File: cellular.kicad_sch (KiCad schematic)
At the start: 50 parts, among them J5 SIM8060-6-1-14-00-A, J6 Conn_Coaxial, J7 Conn_Coaxial, Q6 MMBT3904, Q7 MMBT3904, U24 SN74AXC4T245QPWRQ1, U25 SN74AXC4T245QPWRQ1, U26 BG95-M3

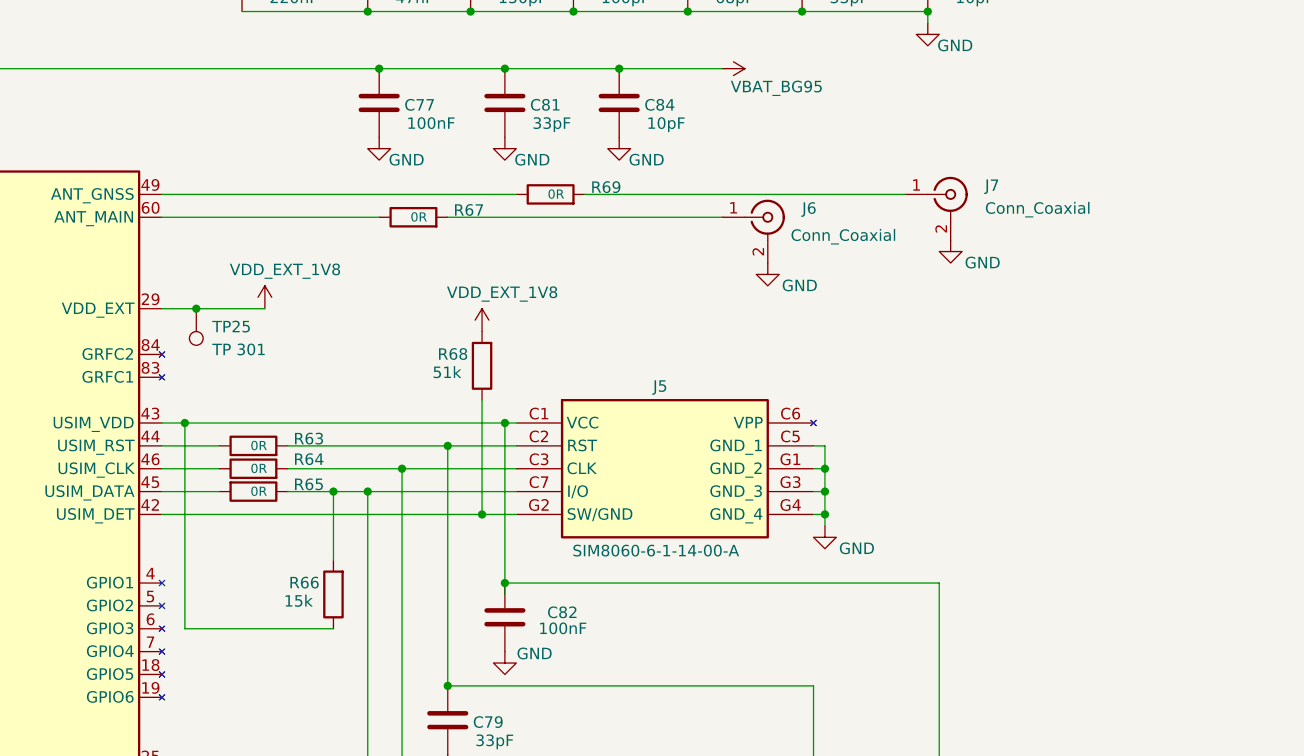
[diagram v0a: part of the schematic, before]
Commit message: bug fix
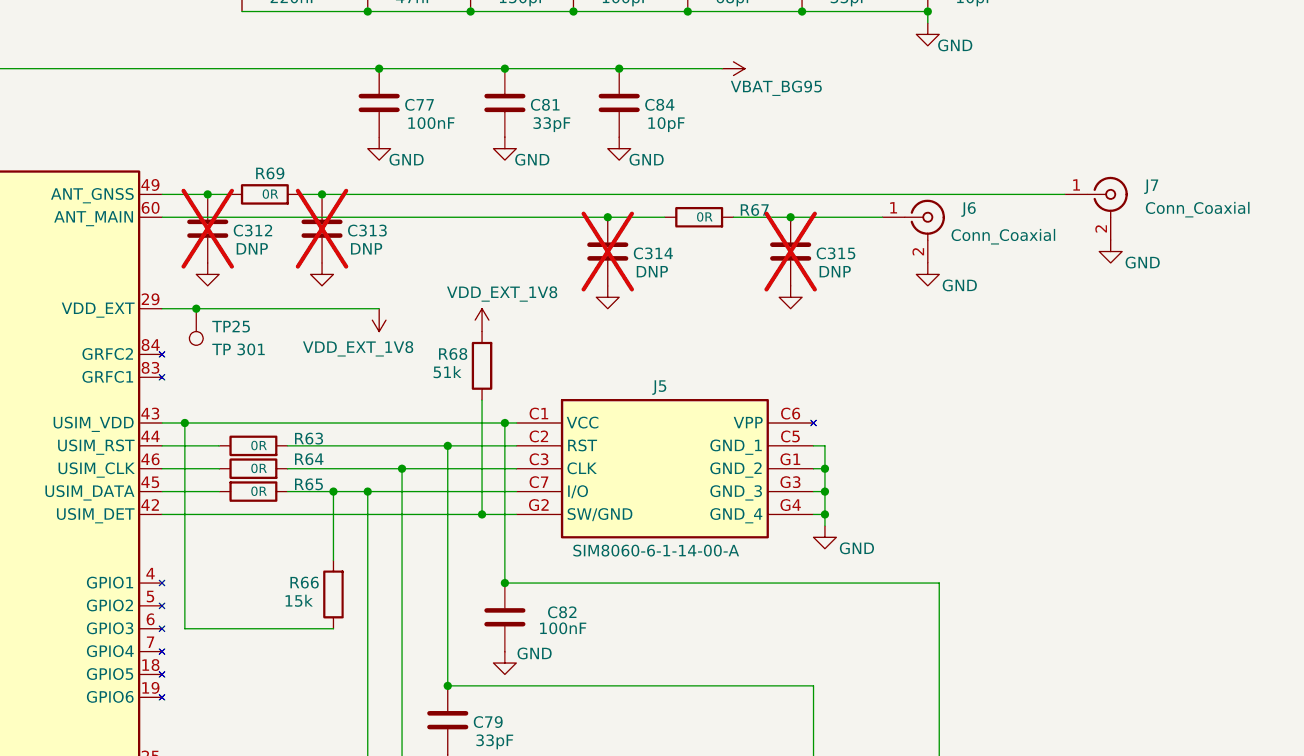
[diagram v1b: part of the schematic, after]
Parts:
- added C312, C313, C314, C315: DNP, RF_Module:ESP32-C6-MINI-1, symbol Device:C
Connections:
- net GND: now also C312.1, C313.1, C314.1, C315.1
- net at R69.1, U26.49 (ANT_GNSS): now also C312.2
- net at R67.1, U26.60 (ANT_MAIN): now also C314.2
- net at J6.1 (In), R67.2: now also C315.2
- net at J7.1 (In), R69.2: now also C313.2
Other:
- moved on the sheet: J6, J7, R67, R69

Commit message: Footprint
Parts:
- FB1: footprint (none) -> Inductor_SMD:L_0402_1005Metric
- J5: footprint SIM8060611400A -> SamacSys_Parts:SIM8060611400A
- J6, J7: footprint (none) -> Connector_Coaxial:U.FL_Hirose_U.FL-R-SMT-1_Vertical
- Q6, Q7: footprint SOT95P230X110-3N -> SamacSys_Parts:SOT95P230X110-3N
- R59, R60, R61, R62, R63, R64, R65, R66, R67, R68, R69: footprint (none) -> Resistor_SMD:R_0402_1005Metric
- TP18, TP19, TP20, TP21, TP22, TP23, TP24, TP25: footprint SOT95P230X110-3N -> TestPoint:TestPoint_Pad_D1.5mm
- U24, U25: footprint SOP65P640X120-16N -> SamacSys_Parts:SOP65P640X120-16N
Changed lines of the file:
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@@
 			)
 		)
-		(property "Footprint" "SOP65P640X120-16N"
+		(property "Footprint" "SamacSys_Parts:SOP65P640X120-16N"
 			(at 78.74 206.68 0)
 			(hide yes)
@@
 			)
 		)
-		(property "Footprint" ""
+		(property "Footprint" "Resistor_SMD:R_0402_1005Metric"
 			(at 163.83 80.518 90)
 			(hide yes)
@@
 			)
 		)
-		(property "Footprint" "SOT95P230X110-3N"
+		(property "Footprint" "SamacSys_Parts:SOT95P230X110-3N"
 			(at -8.56 54.61 0)
 			(hide yes)
@@
 			)
 		)
-		(property "Footprint" "SOT95P230X110-3N"
+		(property "Footprint" "SamacSys_Parts:SOT95P230X110-3N"
 			(at -21.26 35.56 0)
 			(hide yes)
@@
 			)
 		)
-		(property "Footprint" "SOT95P230X110-3N"
+		(property "Footprint" "TestPoint:TestPoint_Pad_D1.5mm"
 			(at 93.98 160.02 0)
 			(hide yes)
@@
 			)
 		)
-		(property "Footprint" ""
+		(property "Footprint" "Resistor_SMD:R_0402_1005Metric"
 			(at 66.548 26.67 90)
 			(hide yes)
@@
 			)
 		)
-		(property "Footprint" ""
+		(property "Footprint" "Inductor_SMD:L_0402_1005Metric"
 			(at 257.81 22.098 90)
 			(hide yes)
@@
 			)
 		)
-		(property "Footprint" ""
+		(property "Footprint" "Resistor_SMD:R_0402_1005Metric"
 			(at 163.83 79.502 90)
 			(hide yes)
@@
 			)
 		)
-		(property "Footprint" "SOT95P230X110-3N"
+		(property "Footprint" "TestPoint:TestPoint_Pad_D1.5mm"
 			(at 93.98 163.83 0)
 			(hide yes)
@@
 			)
 		)
-		(property "Footprint" "SIM8060611400A"
+		(property "Footprint" "SamacSys_Parts:SIM8060611400A"
 			(at 222.25 168.58 0)
 			(hide yes)
@@
 			)
 		)
-		(property "Footprint" "SOT95P230X110-3N"
+		(property "Footprint" "TestPoint:TestPoint_Pad_D1.5mm"
 			(at 152.4 60.96 0)
 			(hide yes)
@@
 			)
 		)
-		(property "Footprint" ""
+		(property "Footprint" "Resistor_SMD:R_0402_1005Metric"
 			(at 191.008 67.31 90)
 			(hide yes)
@@
 			)
 		)
-		(property "Footprint" "SOT95P230X110-3N"
+		(property "Footprint" "TestPoint:TestPoint_Pad_D1.5mm"
 			(at 93.98 148.59 0)
 			(hide yes)
@@
 			)
 		)
-		(property "Footprint" ""
+		(property "Footprint" "Resistor_SMD:R_0402_1005Metric"
 			(at 55.88 23.368 90)
 			(hide yes)
@@
 			)
 		)
-		(property "Footprint" "SOP65P640X120-16N"
+		(property "Footprint" "SamacSys_Parts:SOP65P640X120-16N"
 			(at 78.74 158.42 0)
 			(hide yes)
@@
 			)
 		)
-		(property "Footprint" ""
+		(property "Footprint" "Connector_Coaxial:U.FL_Hirose_U.FL-R-SMT-1_Vertical"
 			(at 238.76 50.8 0)
 			(hide yes)
@@
 			)
 		)
-		(property "Footprint" ""
+		(property "Footprint" "Resistor_SMD:R_0402_1005Metric"
 			(at 213.36 52.578 90)
 			(hide yes)
@@
 			)
 		)
-		(property "Footprint" ""
+		(property "Footprint" "Resistor_SMD:R_0402_1005Metric"
 			(at 55.88 42.418 90)
 			(hide yes)
@@
 			)
 		)
-		(property "Footprint" "SOT95P230X110-3N"
+		(property "Footprint" "TestPoint:TestPoint_Pad_D1.5mm"
 			(at 93.98 156.21 0)
 			(hide yes)
@@
 			)
 		)
-		(property "Footprint" ""
+		(property "Footprint" "Connector_Coaxial:U.FL_Hirose_U.FL-R-SMT-1_Vertical"
 			(at 259.08 48.26 0)
 			(hide yes)
@@
 			)
 		)
-		(property "Footprint" ""
+		(property "Footprint" "Resistor_SMD:R_0402_1005Metric"
 			(at 165.1 50.038 90)
 			(hide yes)
@@
 			)
 		)
-		(property "Footprint" ""
+		(property "Footprint" "Resistor_SMD:R_0402_1005Metric"
 			(at 174.498 92.71 90)
 			(hide yes)
@@
 			)
 		)
-		(property "Footprint" "SOT95P230X110-3N"
+		(property "Footprint" "TestPoint:TestPoint_Pad_D1.5mm"
 			(at 93.98 152.4 0)
 			(hide yes)
@@
 			)
 		)
-		(property "Footprint" ""
+		(property "Footprint" "Resistor_SMD:R_0402_1005Metric"
 			(at 163.83 77.978 90)
 			(hide yes)
@@
 			)
 		)
-		(property "Footprint" "SOT95P230X110-3N"
+		(property "Footprint" "TestPoint:TestPoint_Pad_D1.5mm"
 			(at 93.98 171.45 0)
 			(hide yes)
@@
 			)
 		)
-		(property "Footprint" "SOT95P230X110-3N"
+		(property "Footprint" "TestPoint:TestPoint_Pad_D1.5mm"
 			(at 93.98 167.64 0)
 			(hide yes)
@@
 			)
 		)
-		(property "Footprint" ""
+		(property "Footprint" "Resistor_SMD:R_0402_1005Metric"
 			(at 69.088 44.45 90)
 			(hide yes)

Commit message: Footprint
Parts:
- C312, C313, C314, C315, C70, C71, C72, C73, C74, C75, C76, C77, C78, C79, C80, C81, C82, C83, C84, C85, C86, C87: footprint RF_Module:ESP32-C6-MINI-1 -> Capacitor_SMD:C_0402_1005Metric
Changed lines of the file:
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@@
 			)
 		)
-		(property "Footprint" "RF_Module:ESP32-C6-MINI-1"
+		(property "Footprint" "Capacitor_SMD:C_0402_1005Metric"
 			(at 159.7152 48.26 0)
 			(hide yes)
@@
 			)
 		)
-		(property "Footprint" "RF_Module:ESP32-C6-MINI-1"
+		(property "Footprint" "Capacitor_SMD:C_0402_1005Metric"
 			(at 178.7652 34.29 0)
 			(hide yes)
@@
 			)
 		)
-		(property "Footprint" "RF_Module:ESP32-C6-MINI-1"
+		(property "Footprint" "Capacitor_SMD:C_0402_1005Metric"
 			(at 192.7352 34.29 0)
 			(hide yes)
@@
 			)
 		)
-		(property "Footprint" "RF_Module:ESP32-C6-MINI-1"
+		(property "Footprint" "Capacitor_SMD:C_0402_1005Metric"
 			(at 200.3552 20.32 0)
 			(hide yes)
@@
 			)
 		)
-		(property "Footprint" "RF_Module:ESP32-C6-MINI-1"
+		(property "Footprint" "Capacitor_SMD:C_0402_1005Metric"
 			(at 177.4952 20.32 0)
 			(hide yes)
@@
 			)
 		)
-		(property "Footprint" "RF_Module:ESP32-C6-MINI-1"
+		(property "Footprint" "Capacitor_SMD:C_0402_1005Metric"
 			(at 172.4152 48.26 0)
 			(hide yes)
@@
 			)
 		)
-		(property "Footprint" "RF_Module:ESP32-C6-MINI-1"
+		(property "Footprint" "Capacitor_SMD:C_0402_1005Metric"
 			(at 44.1452 147.32 0)
 			(hide yes)
@@
 			)
 		)
-		(property "Footprint" "RF_Module:ESP32-C6-MINI-1"
+		(property "Footprint" "Capacitor_SMD:C_0402_1005Metric"
 			(at 205.4352 34.29 0)
 			(hide yes)
@@
 			)
 		)
-		(property "Footprint" "RF_Module:ESP32-C6-MINI-1"
+		(property "Footprint" "Capacitor_SMD:C_0402_1005Metric"
 			(at 82.8548 91.44 0)
 			(hide yes)
@@
 			)
 		)
-		(property "Footprint" "RF_Module:ESP32-C6-MINI-1"
+		(property "Footprint" "Capacitor_SMD:C_0402_1005Metric"
 			(at 188.9252 20.32 0)
 			(hide yes)
@@
 			)
 		)
-		(property "Footprint" "RF_Module:ESP32-C6-MINI-1"
+		(property "Footprint" "Capacitor_SMD:C_0402_1005Metric"
 			(at 224.4852 50.8 0)
 			(hide yes)
@@
 			)
 		)
-		(property "Footprint" "RF_Module:ESP32-C6-MINI-1"
+		(property "Footprint" "Capacitor_SMD:C_0402_1005Metric"
 			(at 163.5252 20.32 0)
 			(hide yes)
@@
 			)
 		)
-		(property "Footprint" "RF_Module:ESP32-C6-MINI-1"
+		(property "Footprint" "Capacitor_SMD:C_0402_1005Metric"
 			(at 179.3748 123.19 0)
 			(hide yes)
@@
 			)
 		)
-		(property "Footprint" "RF_Module:ESP32-C6-MINI-1"
+		(property "Footprint" "Capacitor_SMD:C_0402_1005Metric"
 			(at 177.4952 128.27 0)
 			(hide yes)
@@
 			)
 		)
-		(property "Footprint" "RF_Module:ESP32-C6-MINI-1"
+		(property "Footprint" "Capacitor_SMD:C_0402_1005Metric"
 			(at 186.3852 102.87 0)
 			(hide yes)
@@
 			)
 		)
-		(property "Footprint" "RF_Module:ESP32-C6-MINI-1"
+		(property "Footprint" "Capacitor_SMD:C_0402_1005Metric"
 			(at 190.8048 99.06 0)
 			(hide yes)
@@
 			)
 		)
-		(property "Footprint" "RF_Module:ESP32-C6-MINI-1"
+		(property "Footprint" "Capacitor_SMD:C_0402_1005Metric"
 			(at 213.0552 20.32 0)
 			(hide yes)
@@
 			)
 		)
-		(property "Footprint" "RF_Module:ESP32-C6-MINI-1"
+		(property "Footprint" "Capacitor_SMD:C_0402_1005Metric"
 			(at 239.7252 20.32 0)
 			(hide yes)
@@
 			)
 		)
-		(property "Footprint" "RF_Module:ESP32-C6-MINI-1"
+		(property "Footprint" "Capacitor_SMD:C_0402_1005Metric"
 			(at 44.1452 99.06 0)
 			(hide yes)
@@
 			)
 		)
-		(property "Footprint" "RF_Module:ESP32-C6-MINI-1"
+		(property "Footprint" "Capacitor_SMD:C_0402_1005Metric"
 			(at 82.8548 139.7 0)
 			(hide yes)
@@
 			)
 		)
-		(property "Footprint" "RF_Module:ESP32-C6-MINI-1"
+		(property "Footprint" "Capacitor_SMD:C_0402_1005Metric"
 			(at 225.7552 20.32 0)
 			(hide yes)
@@
 			)
 		)
-		(property "Footprint" "RF_Module:ESP32-C6-MINI-1"
+		(property "Footprint" "Capacitor_SMD:C_0402_1005Metric"
 			(at 204.1652 50.8 0)
 			(hide yes)
